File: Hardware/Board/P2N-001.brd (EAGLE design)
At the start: 72 x 72 mm, 38 parts, among them IC1 4053N, IC2 LTC485N, IC3 74LS07N, IC4 LTC485N, K1 G5V1, T1 2SC1815, X1 HIROSE-DX10LM1-14SE

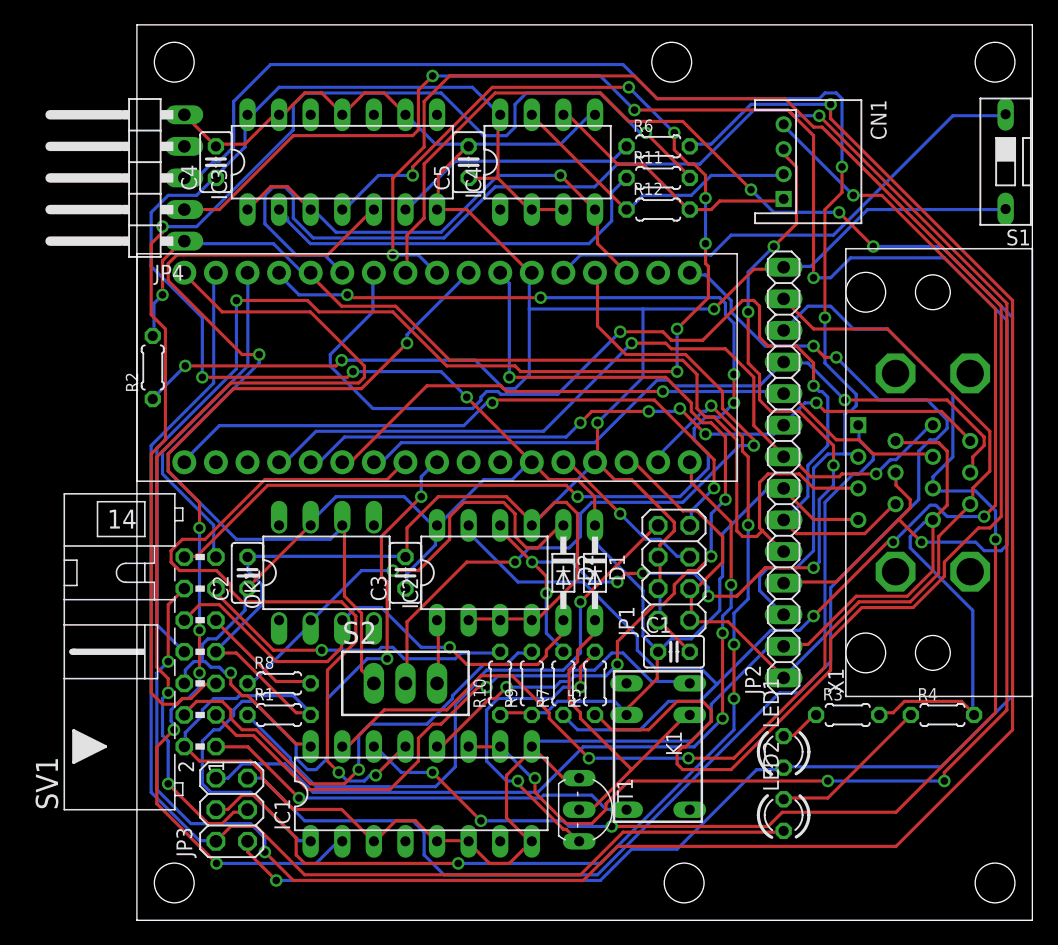
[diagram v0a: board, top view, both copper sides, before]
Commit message: Adopted to XMIDI.
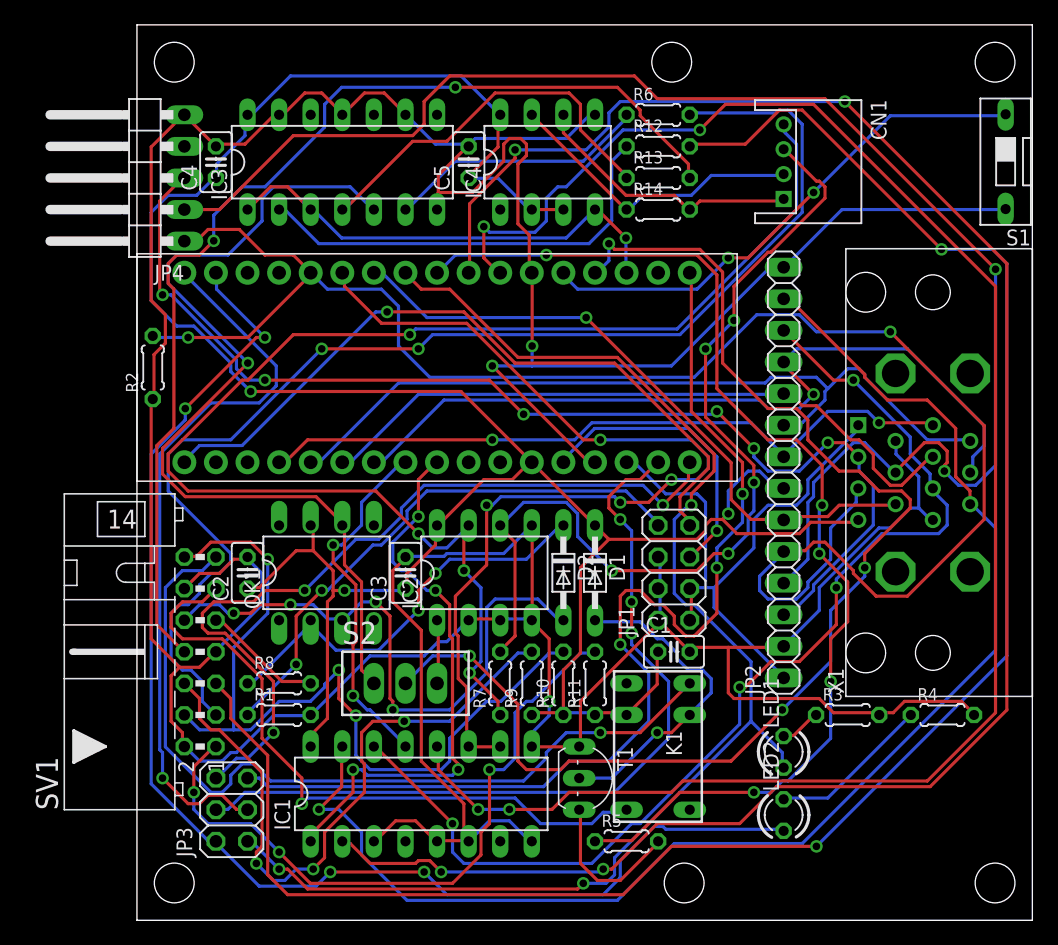
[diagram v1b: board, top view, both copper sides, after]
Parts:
- added R13: 220, resistor:0204/5
- added R14: 120, resistor:0204/5
- R12: value 120 -> 220
- moved R11 41.0 mm to (36.8, 19.1), turned to 90 degrees
- moved R5 13.0 mm to (39.4, 6.35), turned to 0 degrees
- moved R10 5.08 mm to (34.3, 19.1)
- moved R12 5.08 mm to (41.9, 62.2)
- moved R7 5.08 mm to (29.2, 19.1)
- moved R6 2.54 mm to (41.9, 64.8)
- moved T1 2.54 mm to (35.6, 11.4)
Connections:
- removed net CA: K1.5, SV1.1
- removed net CB: K1.10, SV1.3
- removed net N$5: R10.2, SV1.11
- removed net RAWTX: IC3.4, SV1.8
- removed net RETURN: R11.2, SV1.5
- removed net SEND: R9.2, SV1.4
- new net RXRETURN: R6.2, SV1.3
- new net RXSEND: R11.2, SV1.1
- new net TXRETURN: R13.2, SV1.8
- new net TXRETURNII: R12.2, SV1.5
- new net TXSEND: R9.2, SV1.6
- new net TXSENDZV: R10.2, SV1.14, SV1.4
- new net ZVA: K1.5, SV1.11
- new net ZVB: K1.10, SV1.13
- net GND: now also SV1.12
- net N$2: now also R12.1; no longer R11.1
- net N$4: now also IC3.4, R13.1; no longer R6.2, SV1.12
- net SENS0: no longer SV1.13
- net SENS1: no longer SV1.14
- net TX+: now also R14.2; no longer R12.2
- net TX-: now also R14.1; no longer R12.1
- net VCC: now also R11.1; no longer SV1.6
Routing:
- net TXRETURNII: track 0.00 -> 148.6 mm, vias 0 -> 2
- net N$4: track 163.7 -> 30.9 mm, vias 3 -> 0
- net RAWTX: track 124.0 -> 0.00 mm, vias 8 -> 0
- net RXRETURN: track 0.00 -> 103.5 mm, vias 0 -> 2
- net RETURN: track 99.9 -> 0.00 mm, vias 2 -> 0
- net SENS1: track 98.9 -> 0.00 mm, vias 5 -> 0
- net SEL: track 167.2 -> 79.9 mm
- net TXRETURN: track 0.00 -> 86.8 mm, vias 0 -> 2
- net SCL: track 79.3 -> 154.6 mm, vias 6 -> 4
- net SDA: track 68.4 -> 142.6 mm, vias 5 -> 4
- net TXSENDZV: track 0.00 -> 67.3 mm, vias 0 -> 3
- net ZVB: track 0.00 -> 67.0 mm, vias 0 -> 1
- net GPIO0: track 166.4 -> 110.2 mm, vias 4 -> 3
- net RXSEND: track 0.00 -> 54.1 mm, vias 0 -> 3
- net ZVA: track 0.00 -> 53.7 mm, vias 0 -> 1
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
